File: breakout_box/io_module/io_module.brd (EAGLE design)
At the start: 64 x 35 mm, 5 parts, among them U1 AGND, U2 AGND, U3 AGND

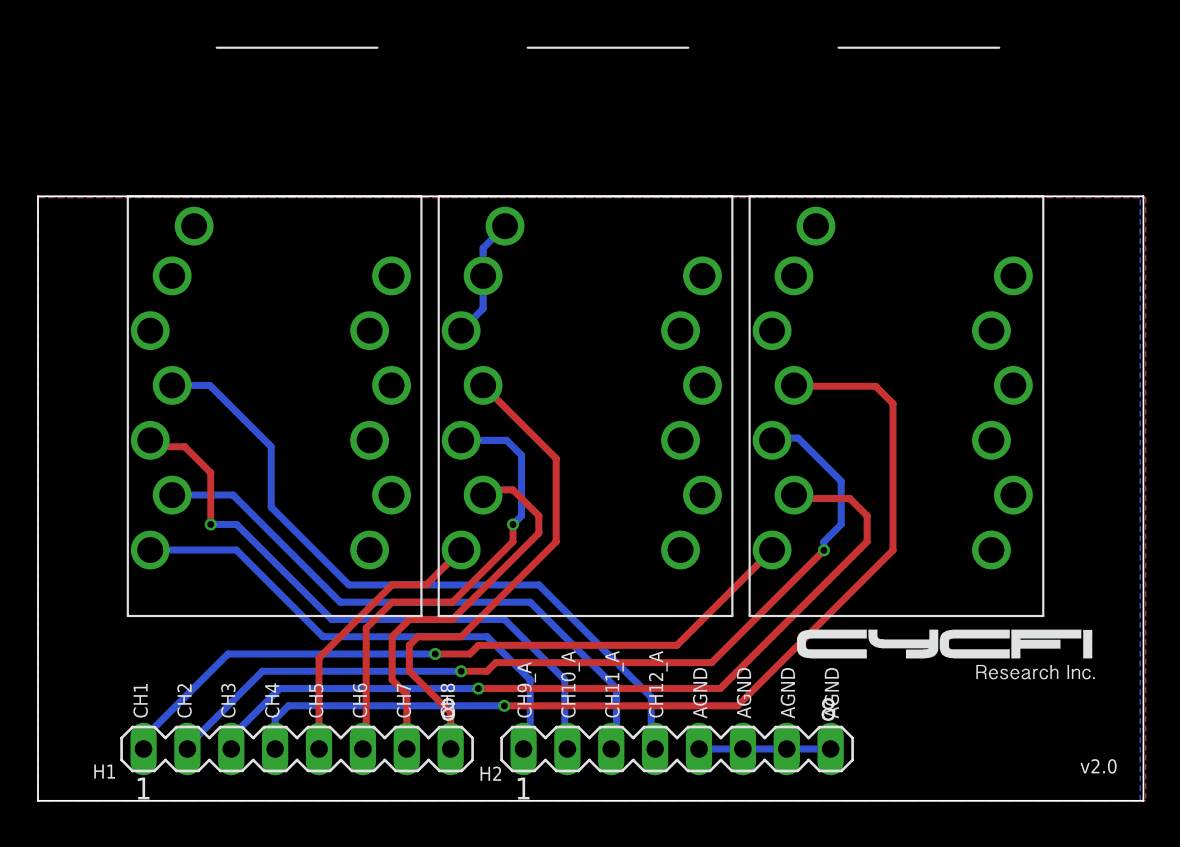
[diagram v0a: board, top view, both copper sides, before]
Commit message: commit and push eagle files for Nexus v2.3
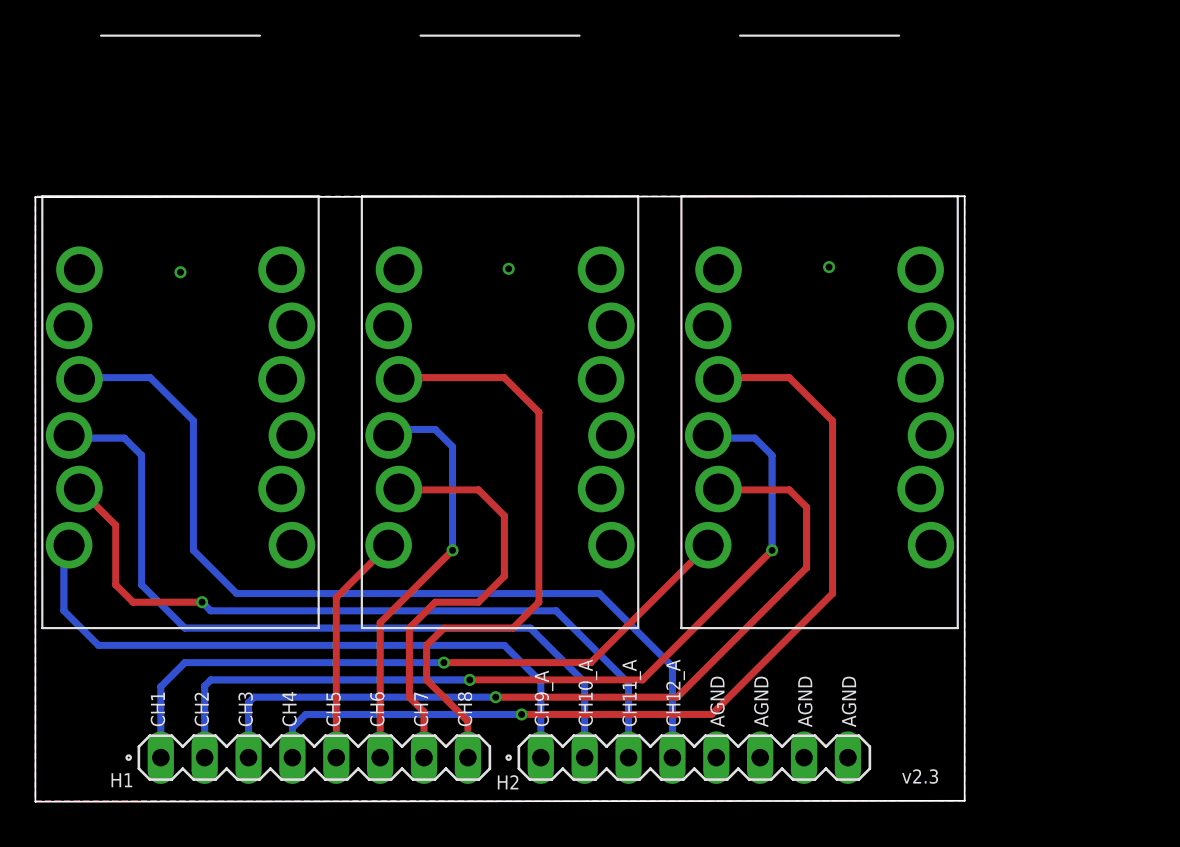
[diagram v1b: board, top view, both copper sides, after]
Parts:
- removed U1, U2, U3: AGND, CYCFI_Jack:NSJ12HC
- added J1, J2, J3: (no value), CYCFI_Jack:ZHEJINAG_CK_6.35
- moved H1 1.12 mm to (16.0, 2.50)
- moved H2 1.12 mm to (38.0, 2.50)
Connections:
- removed net AGND: H2.5, H2.6, H2.7, H2.8, U1.G, U1.SB, U1.ST, U2.G, U2.SB, U2.ST, U3.G, U3.SB, U3.ST
- removed net N$2: H1.2, U1.RT
- new net GND: H2.5, H2.6, H2.7, H2.8, J1.2S, J1.S, J2.2S, J2.S, J3.2S, J3.S
- new net N$13: H1.2, J1.2R
- net N$1: now also J1.2T; no longer U1.TT
- net N$10: now also J3.2R; no longer U3.RT
- net N$11: now also J3.T; no longer U3.TB
- net N$12: now also J3.R; no longer U3.RB
- net N$3: now also J1.T; no longer U1.TB
- net N$4: now also J1.R; no longer U1.RB
- net N$5: now also J2.2T; no longer U2.TT
- net N$6: now also J2.2R; no longer U2.RT
- net N$7: now also J2.T; no longer U2.TB
- net N$8: now also J2.R; no longer U2.RB
- net N$9: now also J3.2T; no longer U3.TT
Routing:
- net N$2: track 51.2 -> 0.00 mm, vias 2 -> 0
- net N$13: track 0.00 -> 49.9 mm, vias 0 -> 2
- net AGND: track 14.7 -> 0.00 mm
- net N$12: track 40.4 -> 51.0 mm
- net N$10: track 35.6 -> 44.5 mm, vias 1 -> 0
- net N$11: track 34.0 -> 42.8 mm, vias 0 -> 1
- net N$9: track 29.3 -> 37.6 mm
- net N$8: track 28.8 -> 35.0 mm
- net N$6: track 26.7 -> 24.0 mm
- net N$5: track 16.1 -> 13.6 mm
- net N$1: track 41.5 -> 39.2 mm
- net N$4: track 56.2 -> 53.9 mm
- net N$7: track 22.8 -> 24.8 mm
- net N$3: track 48.4 -> 47.8 mm
- added copper zone on layer 1, net GND
- added copper zone on layer 16, net GND
- removed copper zone on layer 1, net AGND
- removed copper zone on layer 16, net AGND
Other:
- board size 64 x 35 mm -> 53.8 x 35 mm
- board text added: "v2.3"
- board text removed: "v2.0"
